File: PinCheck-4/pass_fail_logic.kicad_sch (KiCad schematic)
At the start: 6 parts, among them U10 4072, U8 7408, U9 7408

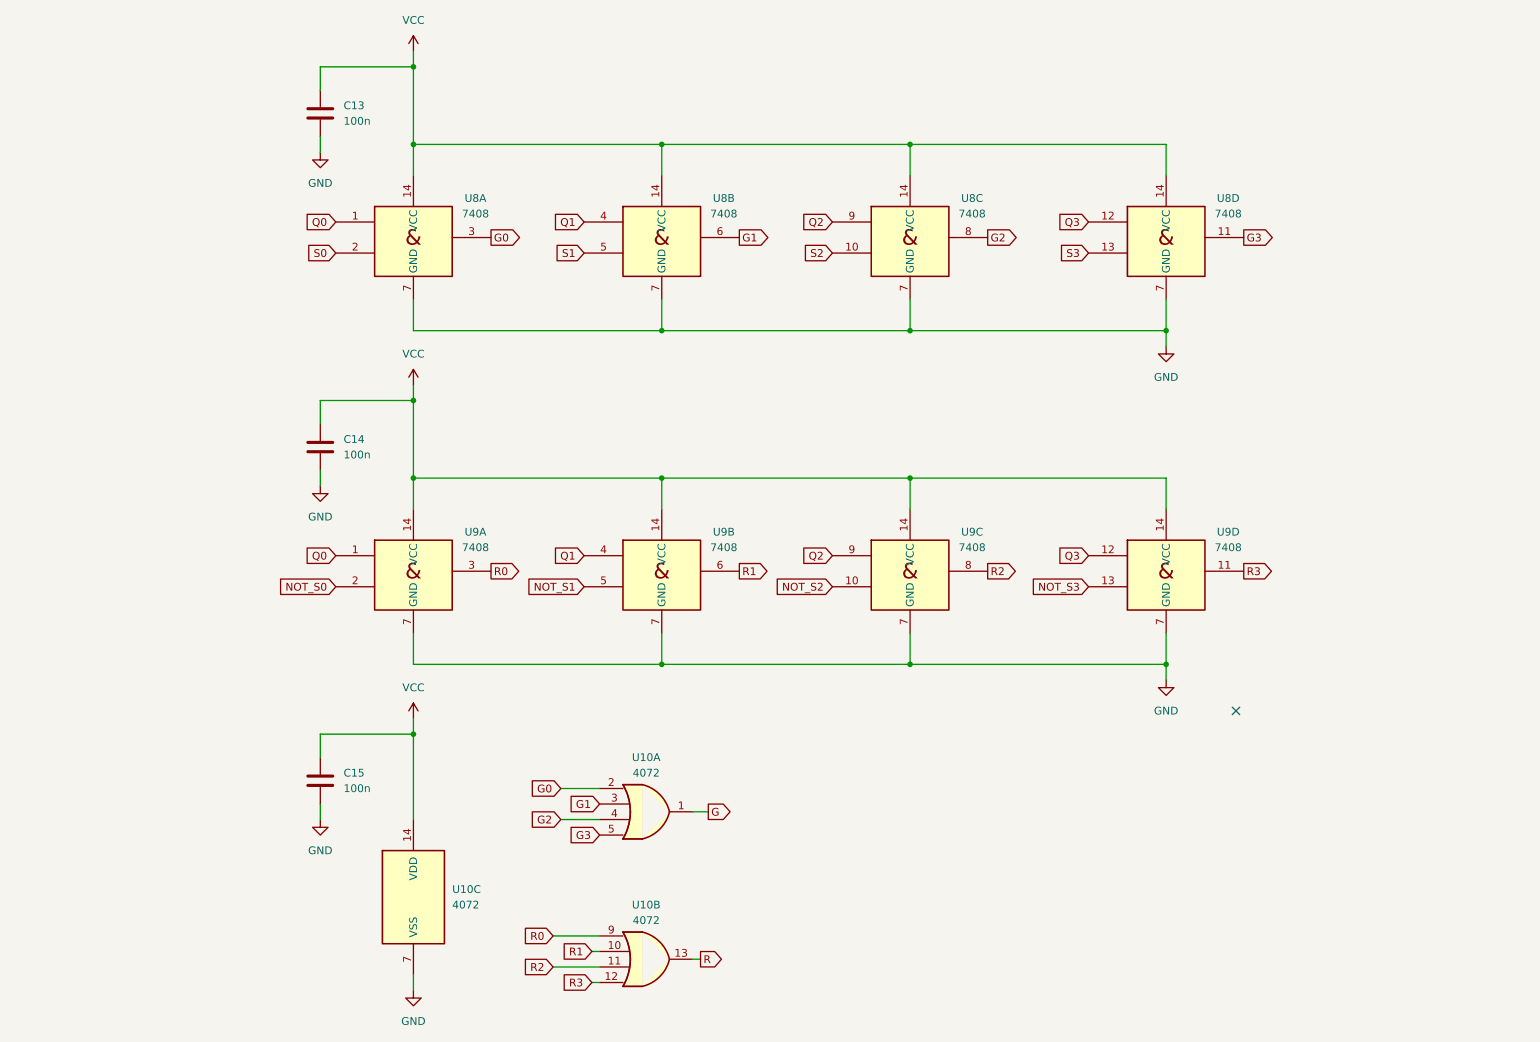
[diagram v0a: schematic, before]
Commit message: Daily sync 2025-08-28 16:55
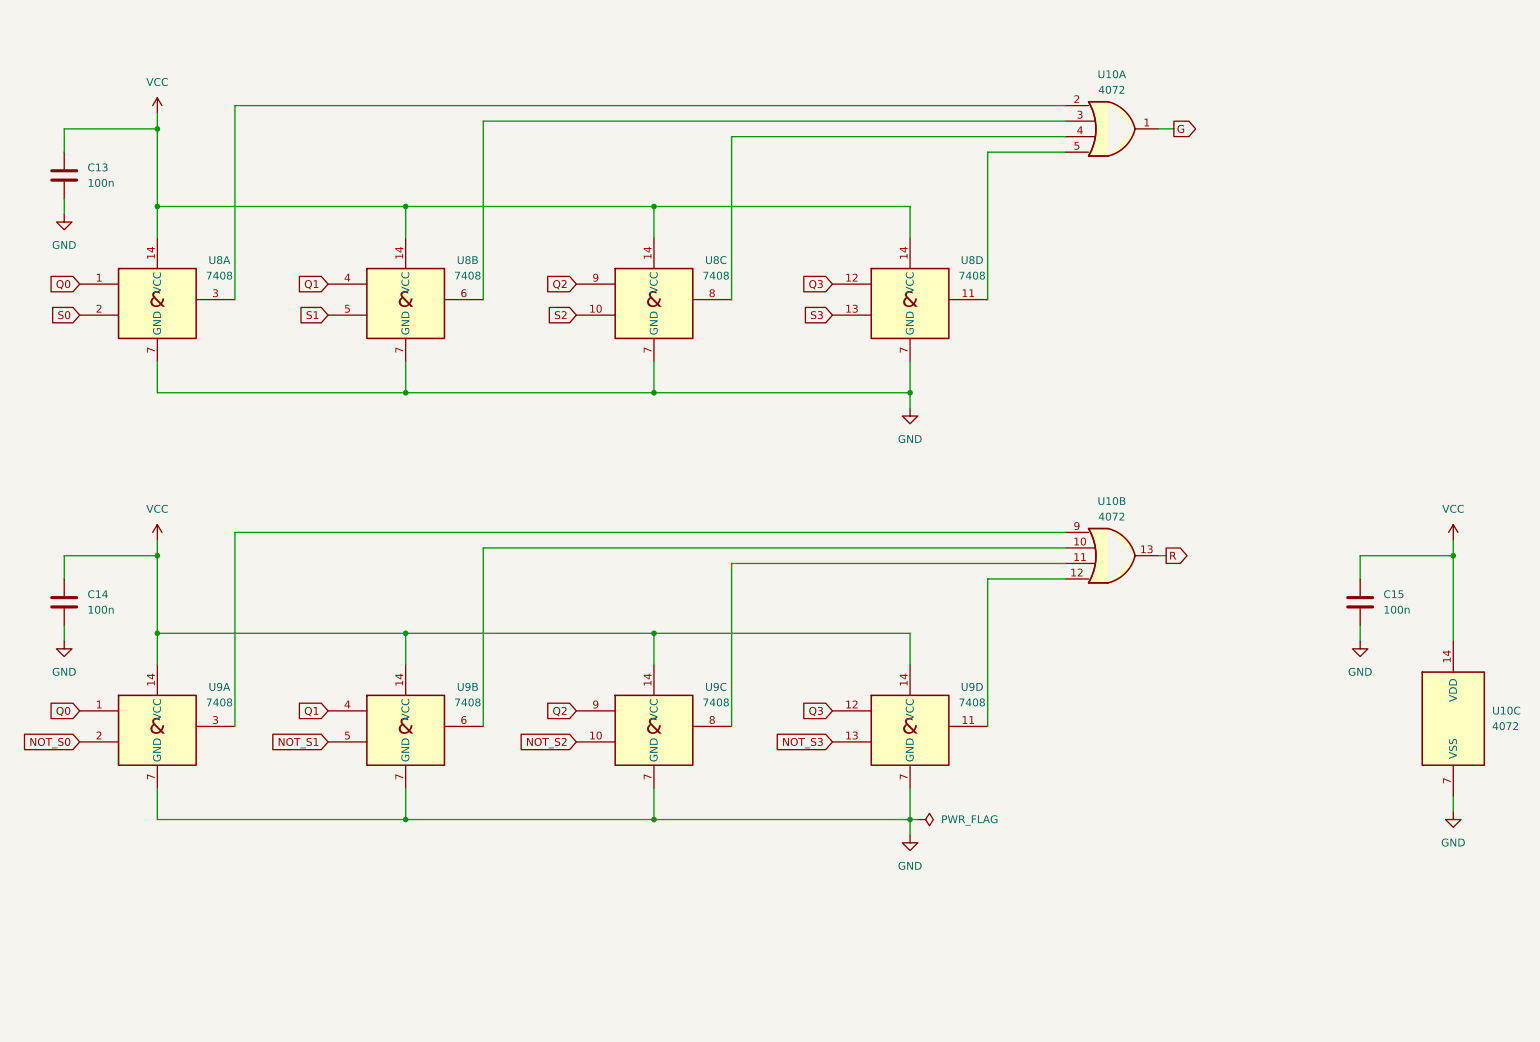
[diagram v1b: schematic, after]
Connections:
- net G0: no longer names the net of U10.2, U8.3
- net G1: no longer names the net of U10.3, U8.6
- net G2: no longer names the net of U10.4, U8.8
- net G3: no longer names the net of U10.5, U8.11
- net R0: no longer names the net of U10.9, U9.3
- net R1: no longer names the net of U10.10, U9.6
- net R2: no longer names the net of U10.11, U9.8
- net R3: no longer names the net of U10.12, U9.11
- no-connect marks 1 -> 0
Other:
- moved on the sheet: C13, C14, C15, U10A, U10B, U10C, U8A, U8B, U8C, U8D, U9A, U9B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

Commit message: Daily sync 2025-08-29 22:48
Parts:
- C13, C14, C15: Manufacturer Part No (none) -> 0805B104K160CT
- U10: Manufacturer Part No (none) -> CD4072BM96
- U8, U9: Manufacturer Part No (none) -> 74HC08D
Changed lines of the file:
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@@
 			)
 		)
-		(property "Description" ""
+		(property "Description" "AND Gate IC 4 Channel 14-SOIC"
+			(at 48.26 130.81 0)
+			(effects
+				(font
+					(size 1.27 1.27)
+				)
+				(hide yes)
+			)
+		)
+		(property "Manufacturer Part No" "74HC08D"
 			(at 48.26 130.81 0)
 			(effects
@@
 			)
 		)
-		(property "Description" ""
+		(property "Description" "AND Gate IC 4 Channel 14-SOIC"
+			(at 171.45 130.81 0)
+			(effects
+				(font
+					(size 1.27 1.27)
+				)
+				(hide yes)
+			)
+		)
+		(property "Manufacturer Part No" "74HC08D"
 			(at 171.45 130.81 0)
 			(effects
@@
 			)
 		)
-		(property "Description" ""
+		(property "Description" "AND Gate IC 4 Channel 14-SOIC"
+			(at 88.9 130.81 0)
+			(effects
+				(font
+					(size 1.27 1.27)
+				)
+				(hide yes)
+			)
+		)
+		(property "Manufacturer Part No" "74HC08D"
 			(at 88.9 130.81 0)
 			(effects
@@
 			)
 		)
-		(property "Description" ""
+		(property "Description" "AND Gate IC 4 Channel 14-SOIC"
+			(at 48.26 60.96 0)
+			(effects
+				(font
+					(size 1.27 1.27)
+				)
+				(hide yes)
+			)
+		)
+		(property "Manufacturer Part No" "74HC08D"
 			(at 48.26 60.96 0)
 			(effects
@@
 			)
 		)
-		(property "Description" "Dual 4 input OR gate"
+		(property "Description" "OR Gate IC 2 Channel 14-SOIC"
+			(at 204.47 33.02 0)
+			(effects
+				(font
+					(size 1.27 1.27)
+				)
+				(hide yes)
+			)
+		)
+		(property "Manufacturer Part No" "CD4072BM96"
 			(at 204.47 33.02 0)
 			(effects
@@
 			)
 		)
-		(property "Description" "Unpolarized capacitor"
+		(property "Description" "SMD Multilayer Ceramic Capacitor, 0.1 µF, 16 V, 0805 [2012 Metric], ± 10%, X7R"
+			(at 245.11 110.49 0)
+			(effects
+				(font
+					(size 1.27 1.27)
+				)
+				(hide yes)
+			)
+		)
+		(property "Manufacturer Part No" "0805B104K160CT"
 			(at 245.11 110.49 0)
 			(effects
@@
 			)
 		)
-		(property "Description" "Dual 4 input OR gate"
+		(property "Description" "OR Gate IC 2 Channel 14-SOIC"
+			(at 260.35 129.54 0)
+			(effects
+				(font
+					(size 1.27 1.27)
+				)
+				(hide yes)
+			)
+		)
+		(property "Manufacturer Part No" "CD4072BM96"
 			(at 260.35 129.54 0)
 			(effects
@@
 			)
 		)
-		(property "Description" ""
+		(property "Description" "AND Gate IC 4 Channel 14-SOIC"
+			(at 129.54 60.96 0)
+			(effects
+				(font
+					(size 1.27 1.27)
+				)
+				(hide yes)
+			)
+		)
+		(property "Manufacturer Part No" "74HC08D"
 			(at 129.54 60.96 0)
 			(effects
@@
 			)
 		)
-		(property "Description" ""
+		(property "Description" "AND Gate IC 4 Channel 14-SOIC"
+			(at 171.45 60.96 0)
+			(effects
+				(font
+					(size 1.27 1.27)
+				)
+				(hide yes)
+			)
+		)
+		(property "Manufacturer Part No" "74HC08D"
 			(at 171.45 60.96 0)
 			(effects
@@
 			)
 		)
-		(property "Description" ""
+		(property "Description" "AND Gate IC 4 Channel 14-SOIC"
+			(at 88.9 60.96 0)
+			(effects
+				(font
+					(size 1.27 1.27)
+				)
+				(hide yes)
+			)
+		)
+		(property "Manufacturer Part No" "74HC08D"
 			(at 88.9 60.96 0)
 			(effects
@@
 			)
 		)
-		(property "Description" "Unpolarized capacitor"
+		(property "Description" "SMD Multilayer Ceramic Capacitor, 0.1 µF, 16 V, 0805 [2012 Metric], ± 10%, X7R"
+			(at 33.02 40.64 0)
+			(effects
+				(font
+					(size 1.27 1.27)
+				)
+				(hide yes)
+			)
+		)
+		(property "Manufacturer Part No" "0805B104K160CT"
 			(at 33.02 40.64 0)
 			(effects
@@
 			)
 		)
-		(property "Description" "Dual 4 input OR gate"
+		(property "Description" "OR Gate IC 2 Channel 14-SOIC"
+			(at 204.47 102.87 0)
+			(effects
+				(font
+					(size 1.27 1.27)
+				)
+				(hide yes)
+			)
+		)
+		(property "Manufacturer Part No" "CD4072BM96"
 			(at 204.47 102.87 0)
 			(effects
@@
 			)
 		)
-		(property "Description" ""
+		(property "Description" "AND Gate IC 4 Channel 14-SOIC"
+			(at 129.54 130.81 0)
+			(effects
+				(font
+					(size 1.27 1.27)
+				)
+				(hide yes)
+			)
+		)
+		(property "Manufacturer Part No" "74HC08D"
 			(at 129.54 130.81 0)
 			(effects
@@
 			)
 		)
-		(property "Description" "Unpolarized capacitor"
+		(property "Description" "SMD Multilayer Ceramic Capacitor, 0.1 µF, 16 V, 0805 [2012 Metric], ± 10%, X7R"
 			(at 33.02 110.49 0)
 			(effects
+				(font
+					(size 1.27 1.27)
+				)
+				(hide yes)
+			)
+		)
+		(property "Manufacturer Part No" "0805B104K160CT"
+			(at 33.02 110.49 0)
+			(effects
